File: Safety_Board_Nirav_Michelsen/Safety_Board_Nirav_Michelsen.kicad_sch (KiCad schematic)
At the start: 0 parts

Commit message: draft_1
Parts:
- added C1, C2, C3: C, symbol Device:C
- added J1, J4: 430450200, SMV_Connectors:CONN_SD-43045-001_02_MOL, symbol SMV_Custom:430450200
- added J2: 22035035, SMV_Connectors:3pin_CON_22035035_MOL, symbol SMV_Custom:3-pin Mini Molex Spox
- added J3, J6: XT60-M, SMV_Connectors:AMASS_XT60-M, symbol SMV_Custom:XT60-M
- added K1: Fujitsu_FTR-LYCA005x, Relay_THT:Relay_SPDT_Fujitsu_FTR-LYCA005x_FormC_Vertical, symbol Relay:Fujitsu_FTR-LYCA005x
- added Q1: IRLML6344TRPBF, IRLML6344TRPBF:TRANS_IRLML6344TRPBF, symbol SMV_Custom:IRLML6344TRPBF
- added U1: MCP6286T-E/OT, SMV_ICs:SOT-23-5_MC_MCH, symbol SMV_Custom:MCP6286T-E_OT
- added U2: ~, symbol SMV_Custom:STM32_Nucleo_F446RE
- added U3: MCP2562-E-P, Package_DIP:DIP-8_W7.62mm, symbol Interface_CAN_LIN:MCP2562-E-P
- added U4: 74LVC1G08, symbol 74xGxx:74LVC1G08
- added U5: XL1509-5.0, Package_SO:SOIC-8_3.9x4.9mm_P1.27mm, symbol Regulator_Switching:XL1509-5.0
- added U6: LDO40LPU33RY, Package_DFN_QFN:DFN-6-1EP_3x3mm_P0.95mm_EP1.7x2.6mm, symbol Regulator_Linear:LDO40LPU33RY
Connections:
- new net: U1.4 (VIN-), U4.4
- new net: J2.1, Q1.3
- new net: J2.3, Q1.2
- new net: U5.5 (GND), U5.6 (GND), U5.7 (GND), U5.8 (GND)
- new net: C2.1, J3.P (POS)
- new net: C1.2, J6.P (POS)
- new net: C3.1, J4.1
- new net: U6.1 (GND), U6.7 (GND)
- new net 12V: C3.2, U1.5 (VDD), U5.2 (OUT), U6.3 (Vin)
- new net 3.3V: J1.1, Q1.1, U2.5 (VDD), U4.2, U6.4 (Vout)
- new net 3.3v: U4.1
- new net 55V: C1.1, C2.2, K1.14, K1.A1, U5.1 (VIN), U5.3 (FB)
- new net CAN_RX: U2.35 (PC2), U3.4 (RXD)
- new net CAN_TX: U2.36 (PC1), U3.1 (TXD)
- new net RELAY_SW: U1.1 (VOUT)

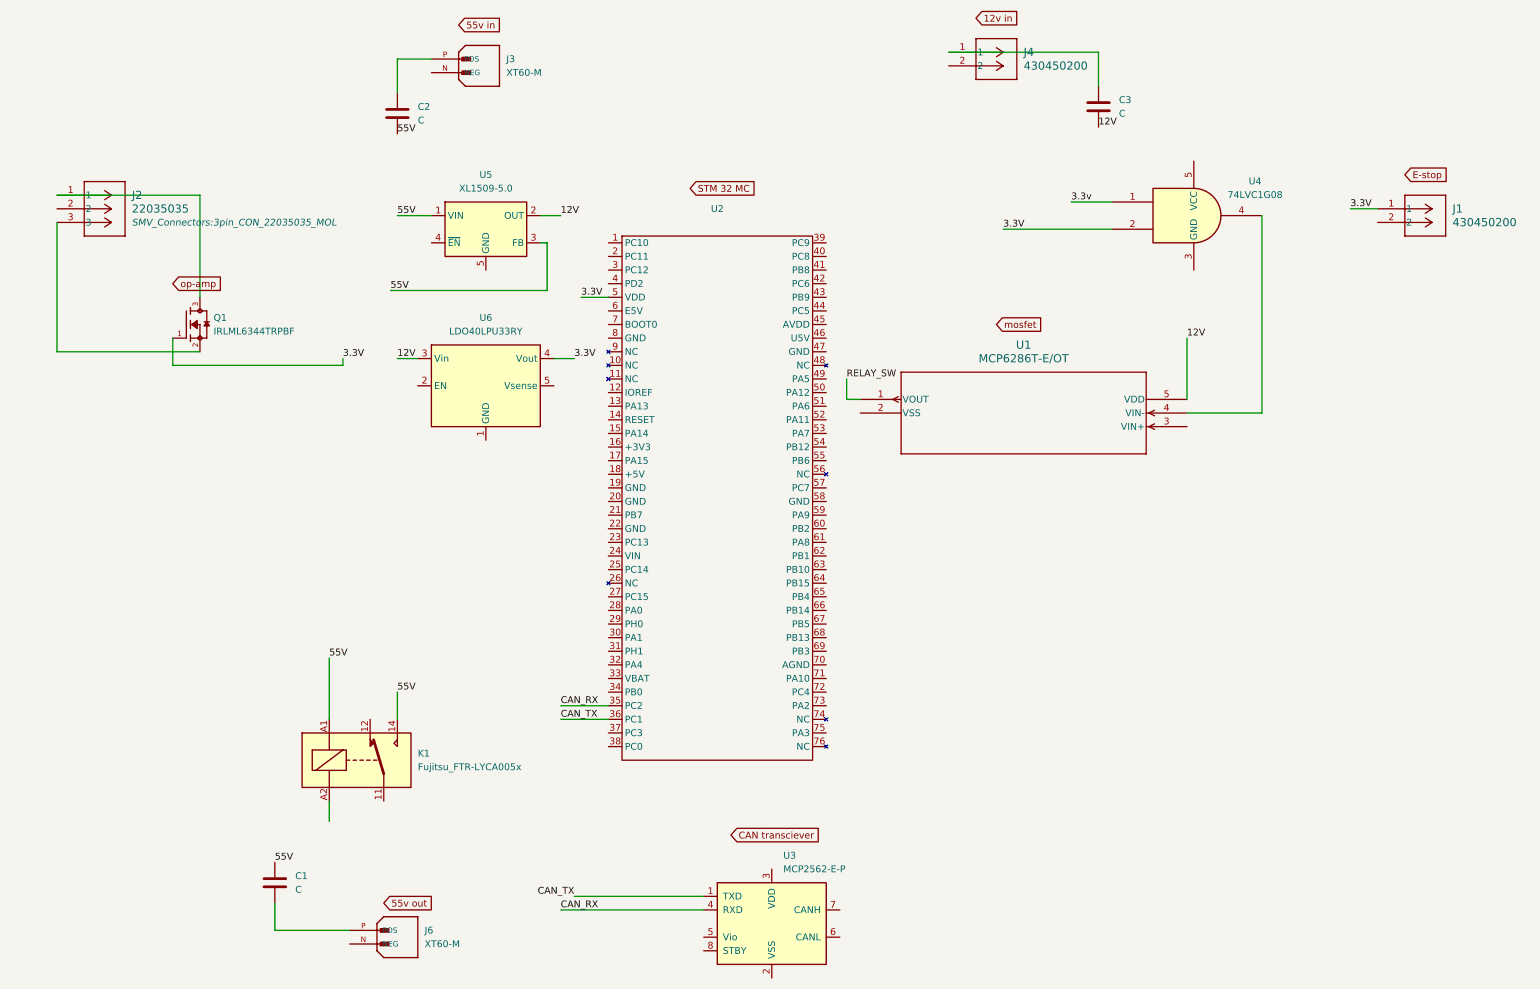
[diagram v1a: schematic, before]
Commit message: draft 2
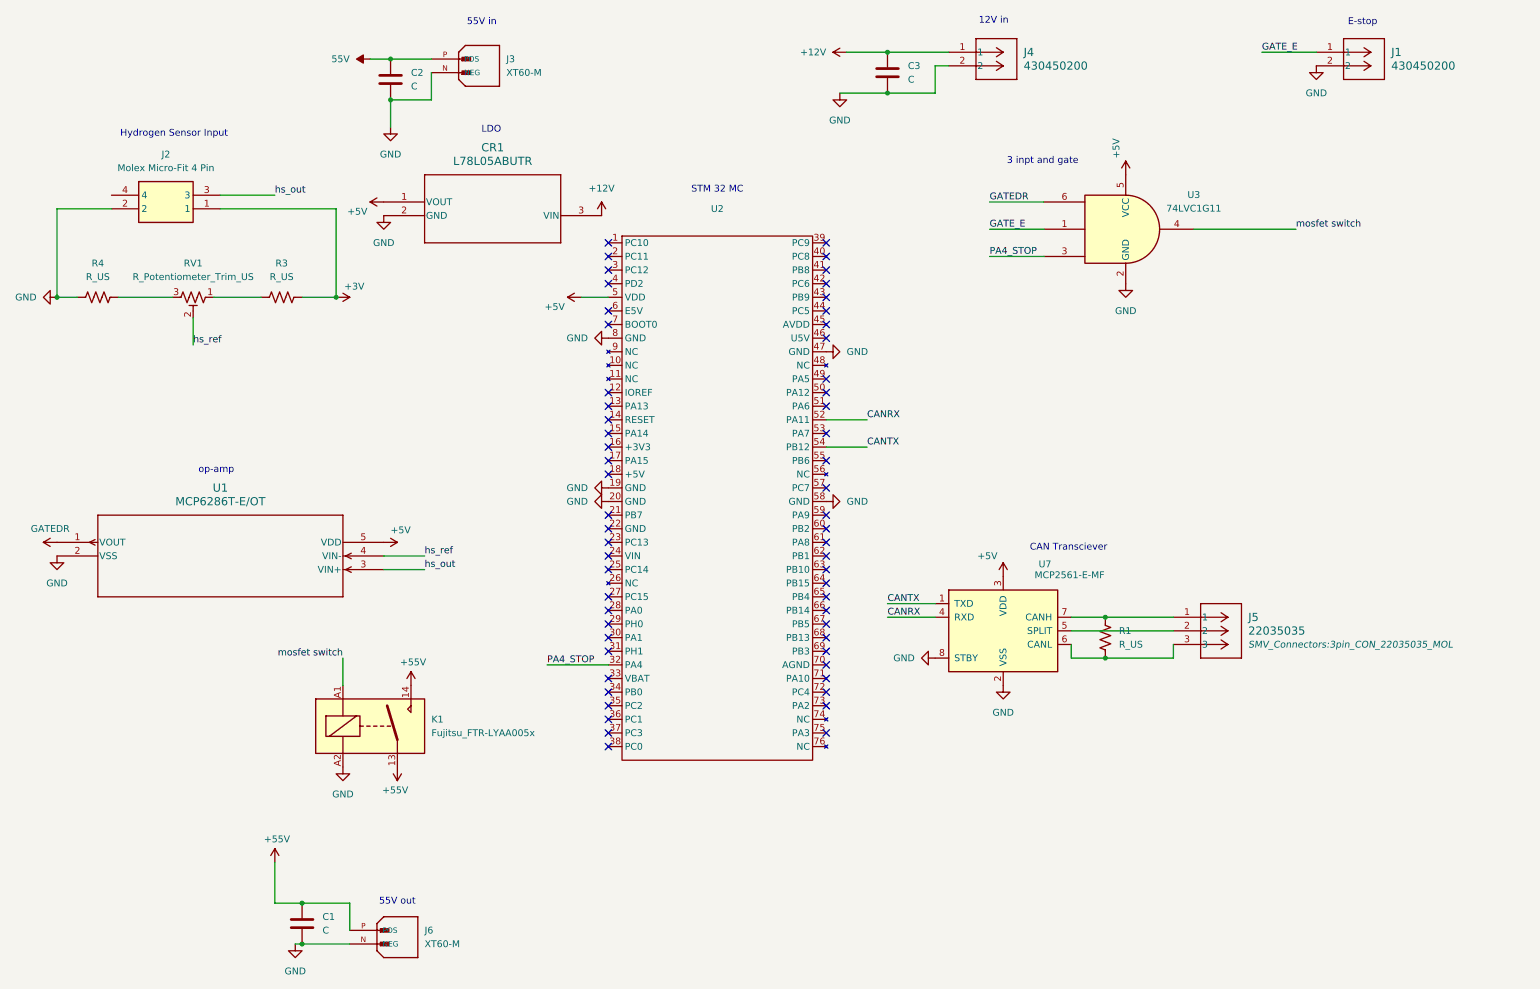
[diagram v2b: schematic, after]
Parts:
- removed J2: 22035035, SMV_Connectors:3pin_CON_22035035_MOL, symbol SMV_Custom:3-pin Mini Molex Spox
- removed K1: Fujitsu_FTR-LYCA005x, Relay_THT:Relay_SPDT_Fujitsu_FTR-LYCA005x_FormC_Vertical, symbol Relay:Fujitsu_FTR-LYCA005x
- removed Q1: IRLML6344TRPBF, IRLML6344TRPBF:TRANS_IRLML6344TRPBF, symbol SMV_Custom:IRLML6344TRPBF
- removed U3: MCP2562-E-P, Package_DIP:DIP-8_W7.62mm, symbol Interface_CAN_LIN:MCP2562-E-P
- removed U4: 74LVC1G08, symbol 74xGxx:74LVC1G08
- removed U5: XL1509-5.0, Package_SO:SOIC-8_3.9x4.9mm_P1.27mm, symbol Regulator_Switching:XL1509-5.0
- removed U6: LDO40LPU33RY, Package_DFN_QFN:DFN-6-1EP_3x3mm_P0.95mm_EP1.7x2.6mm, symbol Regulator_Linear:LDO40LPU33RY
- added CR1: L78L05ABUTR, SMV_Passives:SOT-89_STM, symbol SMV_Custom:L78L05ABUTR
- added J2: Molex Micro-Fit 4 Pin, SMV_Connectors:4_pin0430450401, symbol SMV_Custom:Molex Micro-Fit 4 Pin
- added J5: 22035035, SMV_Connectors:3pin_CON_22035035_MOL, symbol SMV_Custom:3-pin Mini Molex Spox
- added K1: Fujitsu_FTR-LYAA005x, Relay_THT:Relay_SPST-NO_Fujitsu_FTR-LYAA005x_FormA_Vertical, symbol Relay:Fujitsu_FTR-LYAA005x
- added R1, R3, R4: R_US, symbol Device:R_US
- added RV1: R_Potentiometer_Trim_US, symbol Device:R_Potentiometer_Trim_US
- added U3: 74LVC1G11, symbol 74xGxx:74LVC1G11
- added U7: MCP2561-E-MF, Package_DFN_QFN:DFN-8-1EP_3x3mm_P0.65mm_EP1.55x2.4mm, symbol Interface_CAN_LIN:MCP2561-E-MF
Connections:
- net 55V: now also J3.P (POS); no longer C1.1
- net hs_ref: now reaches U1.4 (VIN-)
- net hs_ref: now also RV1.2
- net GND: now reaches J1.2
- net GND: now also C1.2, C2.1, C3.1, J3.N (NEG), J4.2, J6.N (NEG), U1.2 (VSS), U2.19 (GND), U2.20 (GND), U2.47 (GND), U2.58 (GND), U2.8 (GND), CR1.2 (GND), J2.2, K1.A2, R4.1, U3.2 (GND), U7.2 (VSS), U7.8 (STBY), U7.9 (VSS)
- net PA4_STOP: now reaches U2.32 (PA4)
- net PA4_STOP: now also U3.3
- net CANRX: now reaches U2.52 (PA11)
- net CANRX: now also U7.4 (RXD)
- net CANTX: now reaches U2.54 (PB12)
- net CANTX: now also U7.1 (TXD)
- net at U1.3 (VIN+): no longer names the net of U1.3 (VIN+)
- net at U1.3 (VIN+): now also J2.3
- net +55V: now reaches J6.P (POS)
- net +55V: now also C1.1, K1.13, K1.14; no longer C1.2
- net +12V: now reaches J4.1
- net +12V: now also C3.2, CR1.3 (VIN); no longer C3.1
- net 12V renamed +5V
- net +5V: now also U2.5 (VDD), CR1.1 (VOUT), U3.5 (VCC), U7.3 (VDD); no longer C3.2
- net 3.3V renamed GATE_E
- net GATE_E: now also U3.1; no longer U2.5 (VDD)
- net CAN_RX: no longer names the net of U2.35 (PC2)
- net CAN_TX: no longer names the net of U2.36 (PC1)
- net RELAY_SW renamed GATEDR
- net GATEDR: now also U3.6
- new net: J5.1, R1.1, U7.7 (CANH)
- new net: J5.3, R1.2, U7.6 (CANL)
- new net: R3.1, RV1.1
- new net: J5.2, U7.5 (SPLIT)
- new net: R4.2, RV1.3
- new net +3V: J2.1, R3.2
- new net mosfet switch: K1.A1, U3.4
- no-connect marks 0 -> 59
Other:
- note added: "12V in"
- note added: "3 inpt and gate"
- note added: "55V in"
- note added: "55V out"
- note added: "CAN Transciever"
- note added: "E-stop"
- note added: "Hydrogen Sensor Input"
- note added: "LDO"
- note added: "STM 32 MC"
- note added: "op-amp"
- moved on the sheet: C1, C3, J1, U1
